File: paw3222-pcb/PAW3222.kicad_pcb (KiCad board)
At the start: 2 copper layers, 11 x 13 mm, 7 parts, among them J1 Conn_01x06_Socket, U1 PAW3220LU

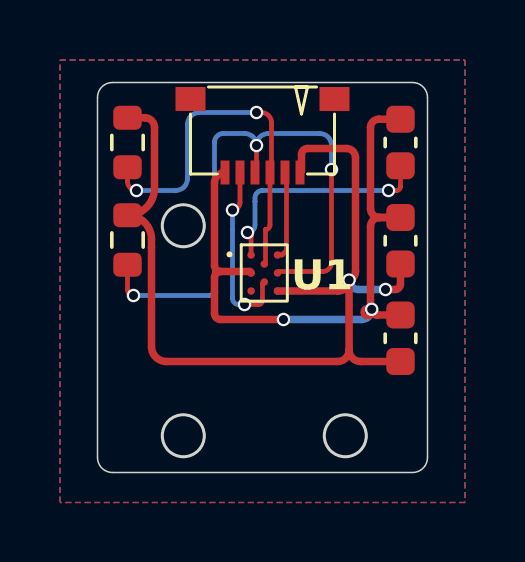
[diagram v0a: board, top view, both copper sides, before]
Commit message: add led
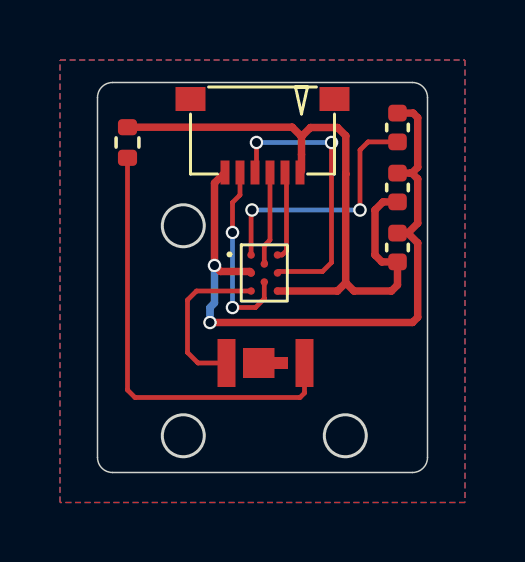
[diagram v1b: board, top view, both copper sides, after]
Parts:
- removed R2: 10kΩ, Resistor_SMD:R_0603_1608Metric
- added D1: IR LED LTE-C216-P-W, paw3222:LTE-C216-P-W, F.Cu at (143.1, 85.8)
- C1, C2, C3: footprint Capacitor_SMD:C_0603_1608Metric -> Capacitor_SMD:C_0402_1005Metric
- R1: value 10kΩ -> 51R; footprint Resistor_SMD:R_0603_1608Metric -> Resistor_SMD:R_0402_1005Metric
- moved C1 3.03 mm to (147.5, 82.0)
- moved C2 1.78 mm to (147.5, 80.0)
- moved C3 0.51 mm to (147.5, 78.0)
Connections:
- R1 pad 1: MOTION -> Net-(D1-A)
- U1 pad E1: unconnected-(U1-LED-PadE1) -> Net-(D1-K)
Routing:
- net Net-(D1-A): track 0.00 -> 14.8 mm
- net SDIO: track 20.3 -> 9.48 mm, vias 3 -> 2
- net VCC 3.3V: track 32.9 -> 22.1 mm, vias 2 -> 0
- net MOTION: track 12.7 -> 3.27 mm, vias 2 -> 0
- net Net-(D1-K): track 0.00 -> 5.44 mm
- net Net-(U1-VDDA): track 7.90 -> 8.53 mm
